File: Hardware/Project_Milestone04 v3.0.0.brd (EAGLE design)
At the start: 134.6 x 107.6 mm, 10 parts, among them IC2 7805T

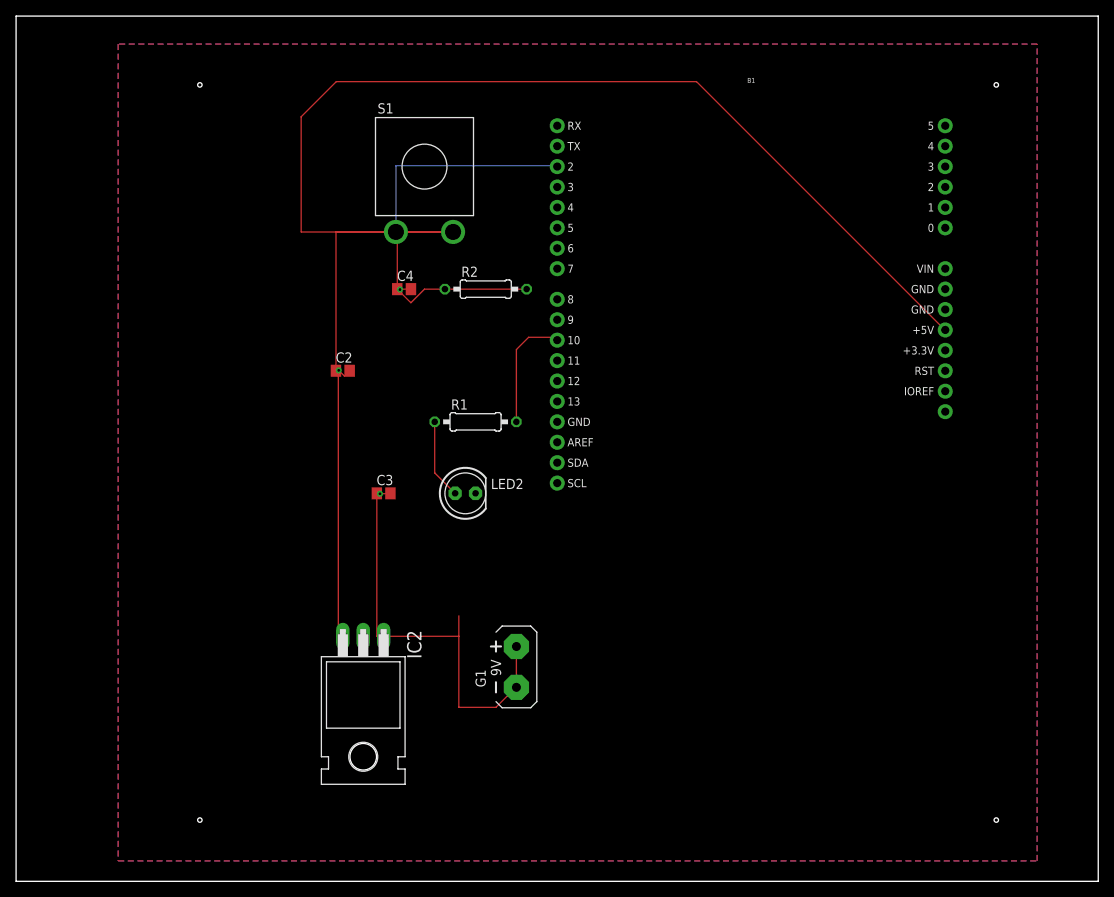
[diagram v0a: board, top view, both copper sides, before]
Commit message: pcb updated
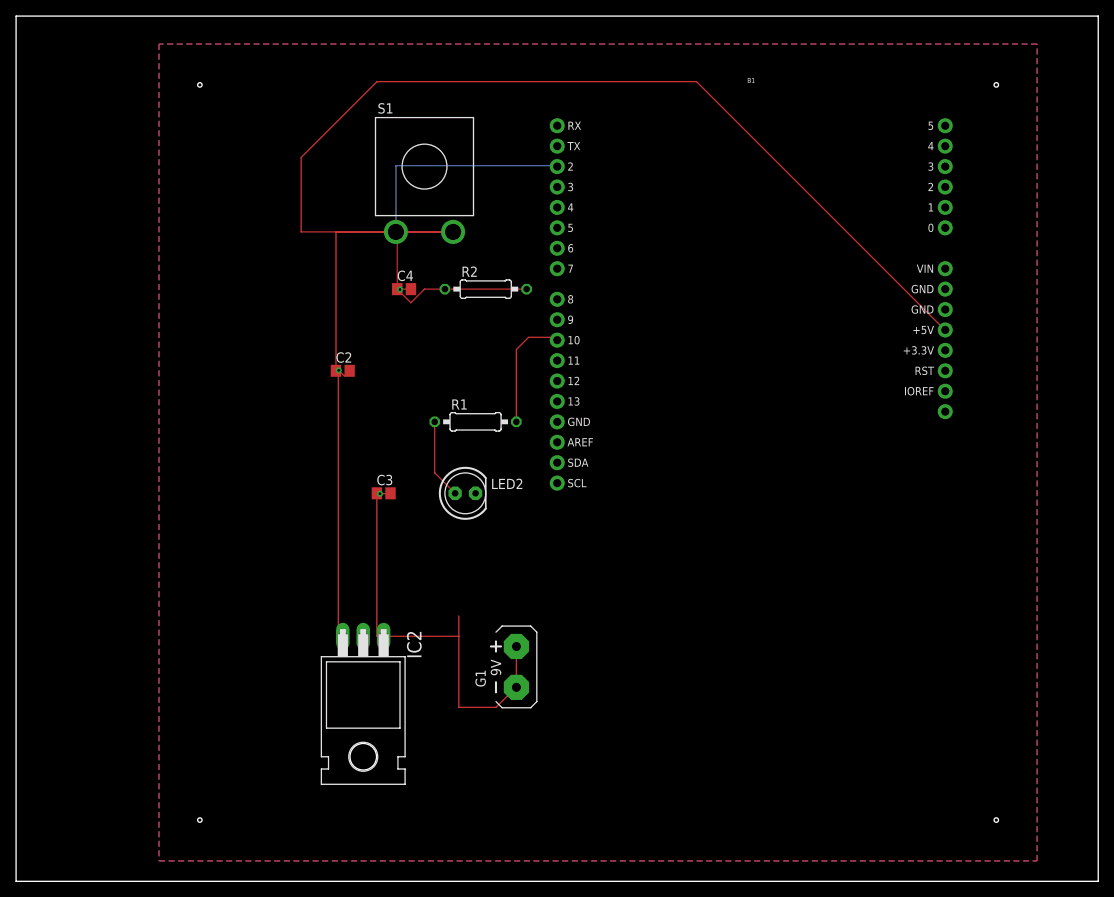
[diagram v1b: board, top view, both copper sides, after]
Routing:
- net VCC: track 193.6 -> 190.6 mm
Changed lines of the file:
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@@
 <drawing>
 <settings>
-<setting alwaysvectorfont="yes"/>
+<setting alwaysvectorfont="no"/>
 <setting verticaltext="up"/>
 </settings>
@@
 <hole x="137.16" y="7.62" drill="0.55"/>
 <hole x="137.16" y="99.06" drill="0.55"/>
+<dimension x1="27.94" y1="104.14" x2="27.94" y2="2.54" x3="142.24" y3="53.34" textsize="1.778" layer="1"/>
+<dimension x1="142.24" y1="2.54" x2="142.24" y2="104.14" x3="27.94" y3="53.34" textsize="1.778" layer="1"/>
 </plain>
 <attributes>
@@
 </variantdefs>
 <classes>
-<class number="0" name="default" width="0" drill="0">
+<class number="0" name="default" width="0.508" drill="0.508">
+<clearance class="0" value="0.508"/>
 </class>
 </classes>
@@
 <contactref element="G1" pad="-"/>
 <polygon width="0.1524" layer="16">
-<vertex x="27.94" y="104.14"/>
-<vertex x="27.94" y="2.54"/>
+<vertex x="33.02" y="104.14"/>
+<vertex x="33.02" y="2.54"/>
 <vertex x="142.24" y="2.54"/>
 <vertex x="142.24" y="104.14"/>
@@
 <wire x1="55.3212" y1="63.407665625" x2="55.03" y2="63.5" width="0.1524" layer="1"/>
 <wire x1="99.8728" y1="99.4664" x2="130.7592" y2="68.58" width="0.1524" layer="1"/>
-<wire x1="99.8728" y1="99.4664" x2="55.0672" y2="99.4664" width="0.1524" layer="1"/>
-<wire x1="55.0672" y1="99.4664" x2="50.6984" y2="95.0976" width="0.1524" layer="1"/>
+<wire x1="99.8728" y1="99.4664" x2="60.1472" y2="99.4664" width="0.1524" layer="1"/>
+<wire x1="60.1472" y1="99.4664" x2="50.6984" y2="90.0176" width="0.1524" layer="1"/>
 <wire x1="130.7592" y1="68.58" x2="130.81" y2="68.58" width="0.1524" layer="1"/>
-<wire x1="50.6984" y1="95.0976" x2="50.6984" y2="80.772" width="0.1524" layer="1"/>
+<wire x1="50.6984" y1="90.0176" x2="50.6984" y2="80.772" width="0.1524" layer="1"/>
 <wire x1="69.596" y1="80.772" x2="50.6984" y2="80.772" width="0.1524" layer="1"/>
 </signal>
 <signal name="TOP">
 <polygon width="0.1524" layer="1">
-<vertex x="27.94" y="104.14"/>
-<vertex x="27.94" y="2.54"/>
+<vertex x="33.02" y="104.14"/>
+<vertex x="33.02" y="2.54"/>
 <vertex x="142.24" y="2.54"/>
 <vertex x="142.24" y="104.14"/>
